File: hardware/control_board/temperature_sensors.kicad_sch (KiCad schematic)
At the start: 24 parts, among them J5 RTD, J5 TC, U2 MAX6675, U5 MCP6N11-005, U7 MCP6001

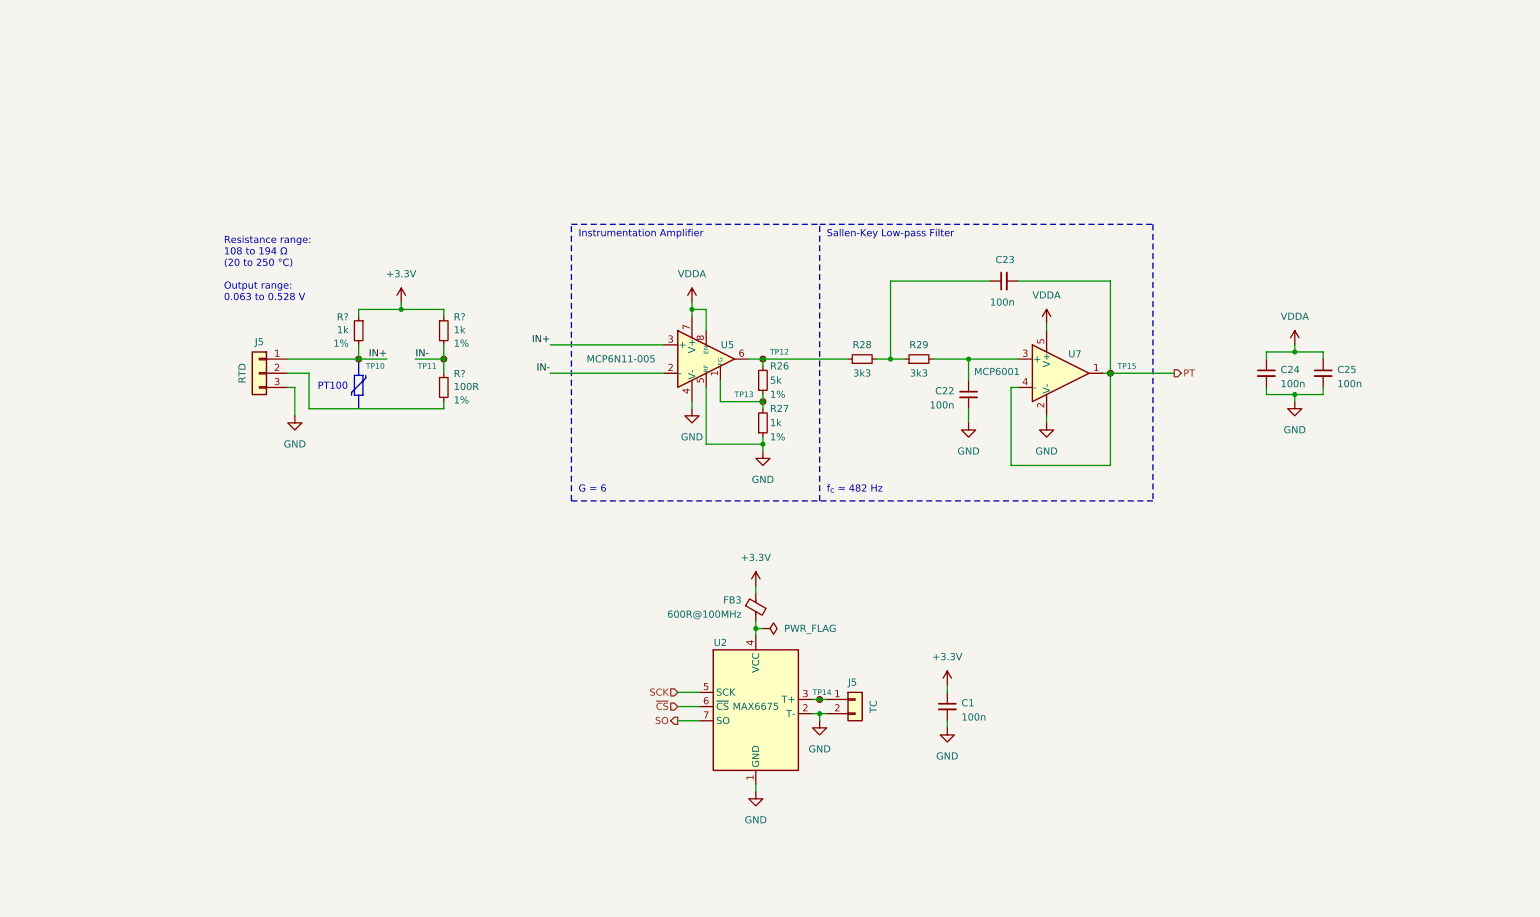
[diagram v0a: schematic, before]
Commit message: Assign footprints to components
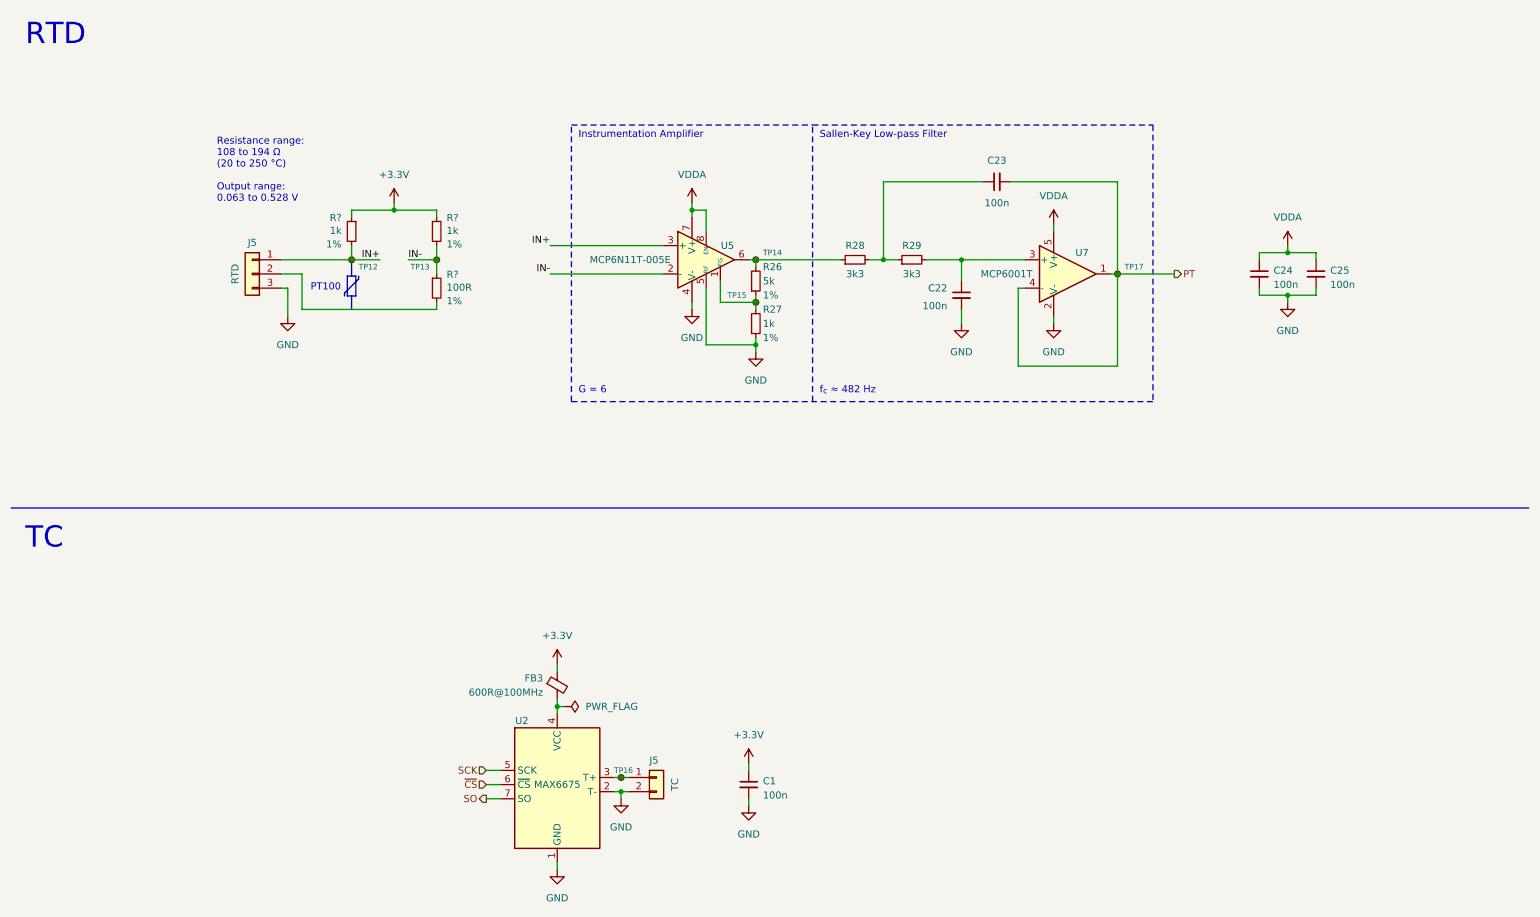
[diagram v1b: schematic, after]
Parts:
- J5: Component (none) -> B3B-XH-A (LF)(SN)
- J5: Component (none) -> B2B-XH-A (LF)(SN)
- U5: value MCP6N11-005 -> MCP6N11T-005E; footprint Package_DFN_QFN:TDFN-8-1EP_3x2mm_P0.5mm_EP1.80x1.65mm -> Package_SO:SOIC-8_3.9x4.9mm_P1.27mm
- U7: value MCP6001 -> MCP6001T
- renumbered TP10 to TP12, TP11 to TP13, TP12 to TP14, TP13 to TP15, TP14 to TP16, TP15 to TP17
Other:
- note added: "RTD"
- note added: "TC"
- moved on the sheet: C1, C22, C23, C24, C25, FB3, J5, R26, R27, R28, R29, R?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
